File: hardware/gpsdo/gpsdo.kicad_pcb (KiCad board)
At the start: 4 copper layers, 70 x 70 mm, 87 parts, among them J1 Conn_01x02, J2 Conn_02x03_Top_Bottom, J3 USB_C_Receptacle_USB2.0_14P, J4 Conn_01x03, J5 Conn_Coaxial, U1 74HC4040D_652, U2 74HC4040D_652, U3 REF5040AD, U4 AD5541A, U5 OPA197xD, U6 STM32F411CEUx, U7 AMS1117-3.3, U9 SN74LVC1G125DBV, X1 X322516MLB4SI

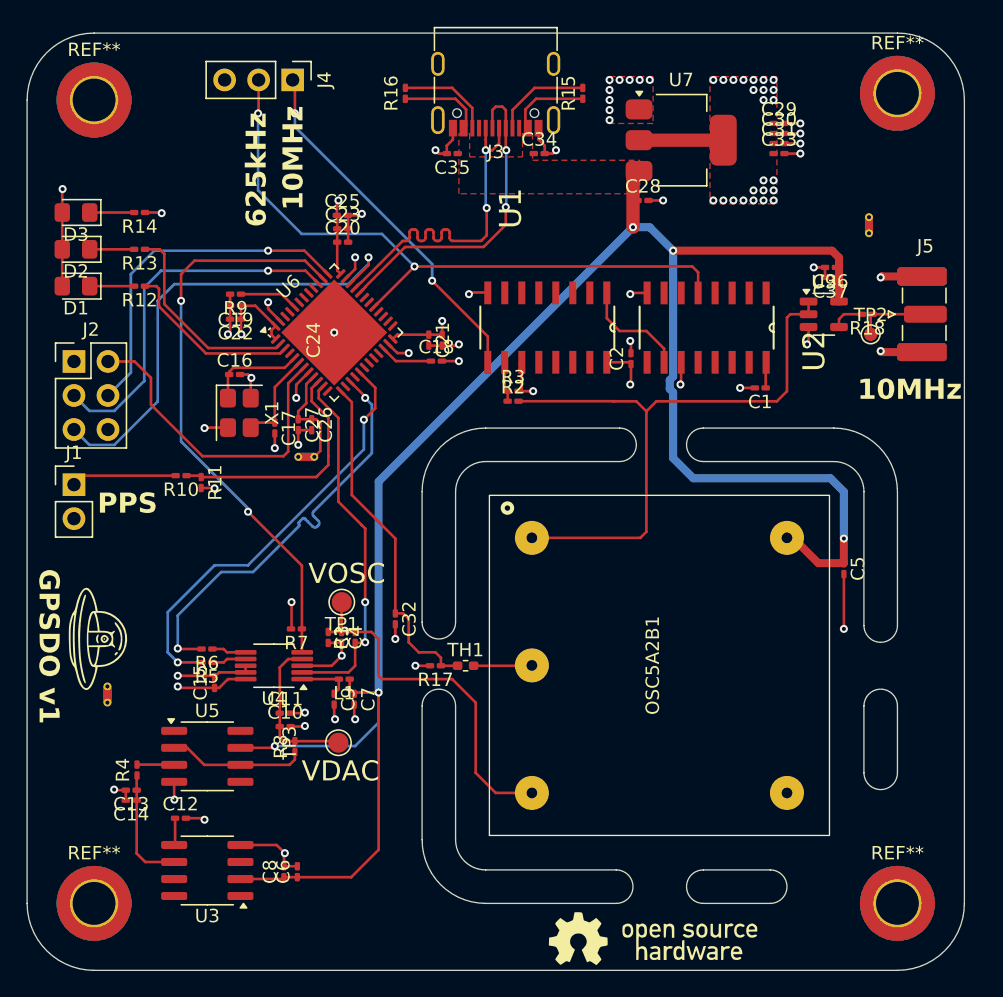
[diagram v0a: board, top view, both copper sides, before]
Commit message: cleanup pcb
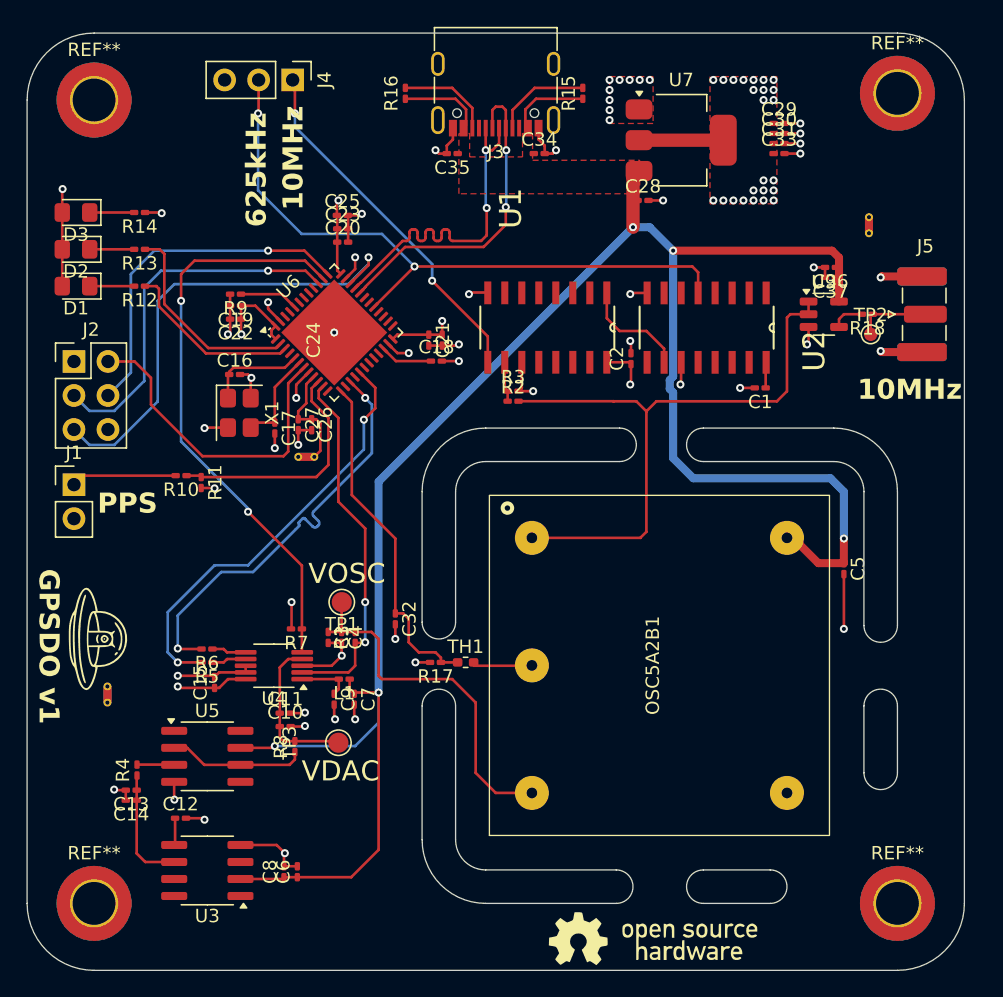
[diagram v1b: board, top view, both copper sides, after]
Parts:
- moved R17 0.25 mm to (138.2, 111.8)
- moved TH1 0.25 mm to (140.5, 111.8)
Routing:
- net GND: track 56.1 -> 54.3 mm
- net VCC_5V: track 158.5 -> 157.0 mm
- net OSC_OUT: track 7.96 -> 6.66 mm
- net VDD_3V3: track 45.4 -> 44.3 mm
- net PPS_5V: track 7.91 -> 6.92 mm
- net OSC_IN: track 7.88 -> 7.19 mm
